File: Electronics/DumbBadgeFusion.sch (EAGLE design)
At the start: 125 parts, among them IC1 SN74CBT16233DGGR, IC2 SN74CBT16233DGGR, SW1 SPST_TACT-KMR2, T1 MMUN2133LT1G, U1 TDP3E001DRLR-SOT-23-5SOT-23-5, U2 TPS61090RSAR, U3 MCP73871, U6 MAX3232, X4 32.768

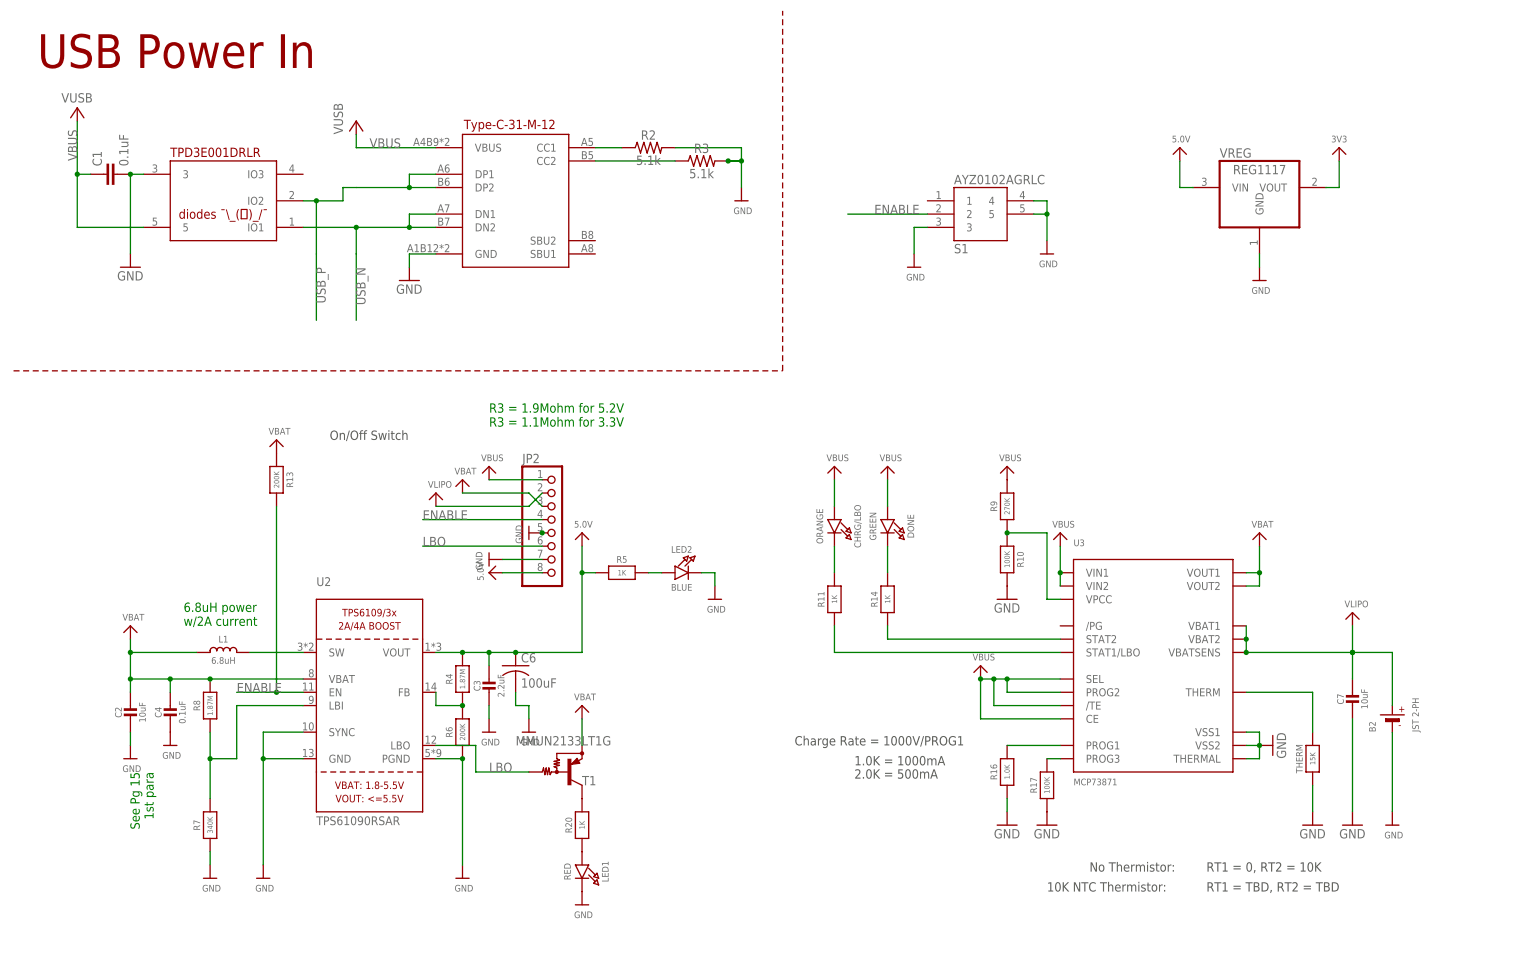
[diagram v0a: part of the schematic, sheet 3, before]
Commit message: more power
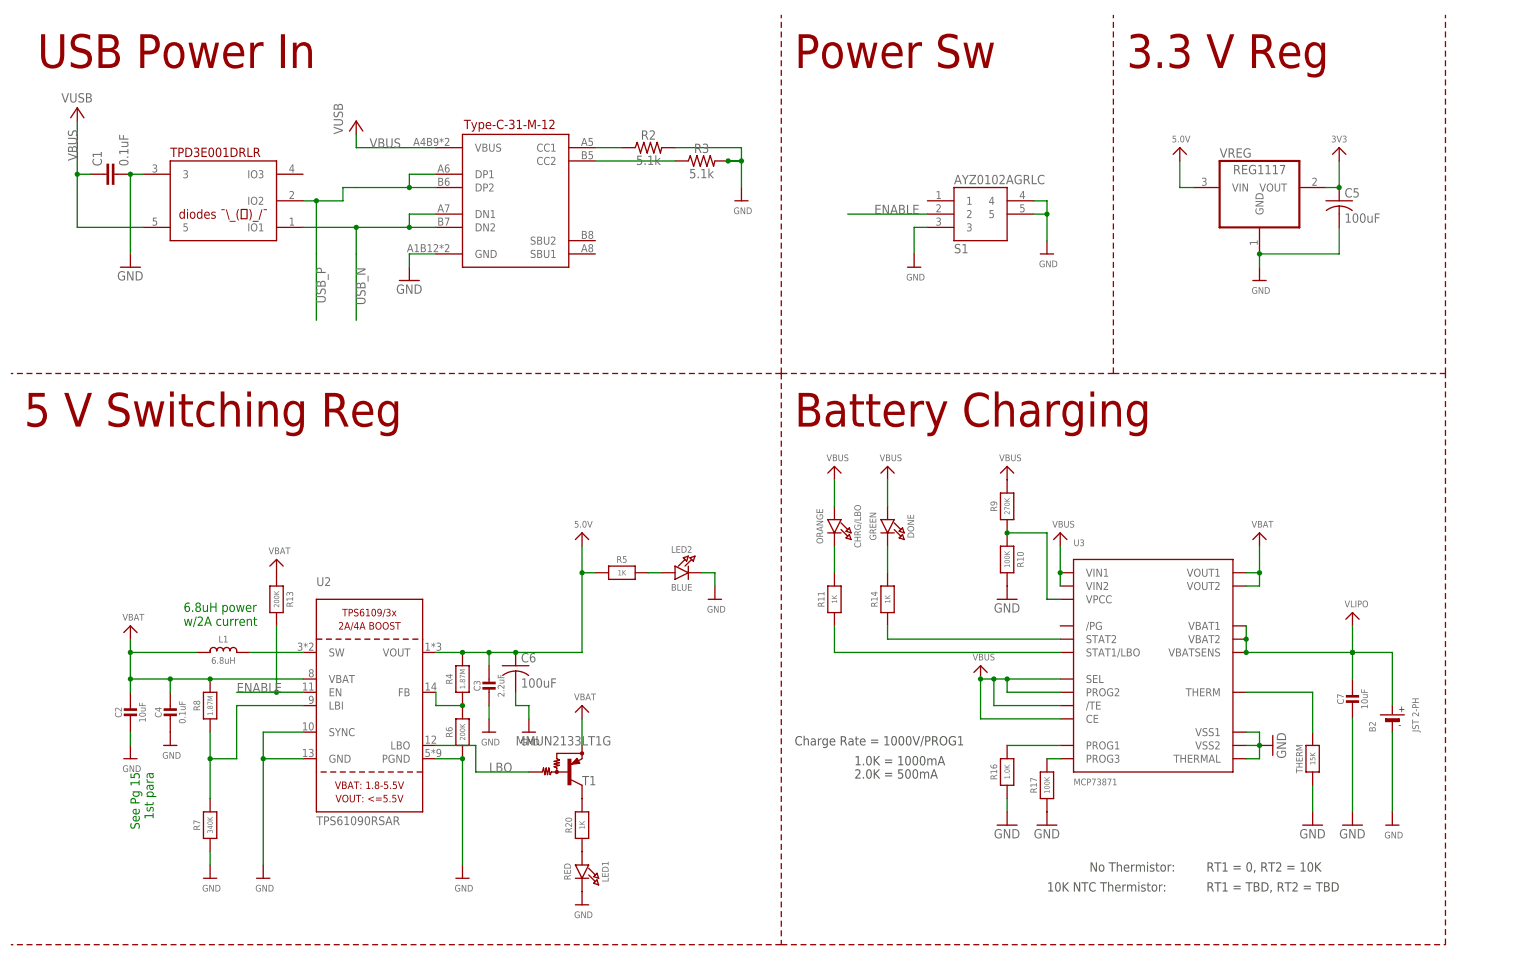
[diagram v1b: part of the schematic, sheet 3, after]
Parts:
- removed JP2: (no value), microbuilder:HEADER-1X8ROUND
- added C5: 100uF, rcl:C-USC1210
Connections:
- net 3V3: now also C5.1
- net 5.0V: no longer JP2.8
- net ENABLE: no longer JP2.4
- net GND: now also C5.2; no longer JP2.5, JP2.7
- net LBO: no longer JP2.6
- net VBAT: no longer JP2.3
- net VBUS: no longer JP2.1
- net VLIPO: no longer JP2.2
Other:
- note added: "3.3 V Reg"
- note added: "5 V Switching Reg"
- note added: "Battery Charging"
- note added: "Power Sw"
- note removed: "On/Off Switch"
- note removed: "R3 = 1.9Mohm for 5.2V R3 = 1.1Mohm for 3.3V"
- moved on the sheet: R13
